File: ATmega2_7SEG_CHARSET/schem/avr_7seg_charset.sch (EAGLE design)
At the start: 19 parts, among them J1 ARDUINO_R3_SHIELD_ICSP-NO_LAB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

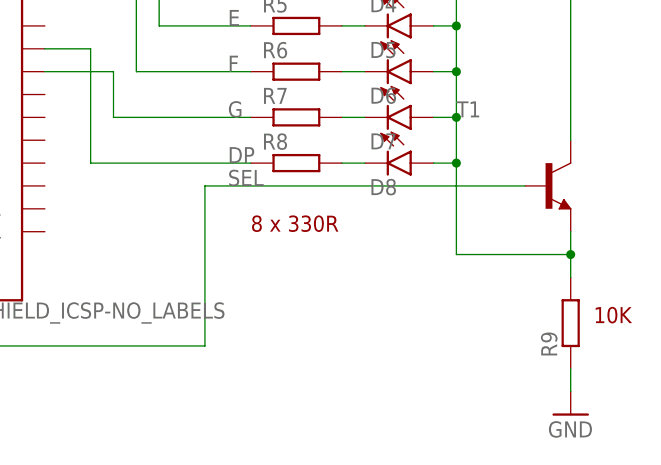
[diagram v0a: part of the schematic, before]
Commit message: corrected the schem
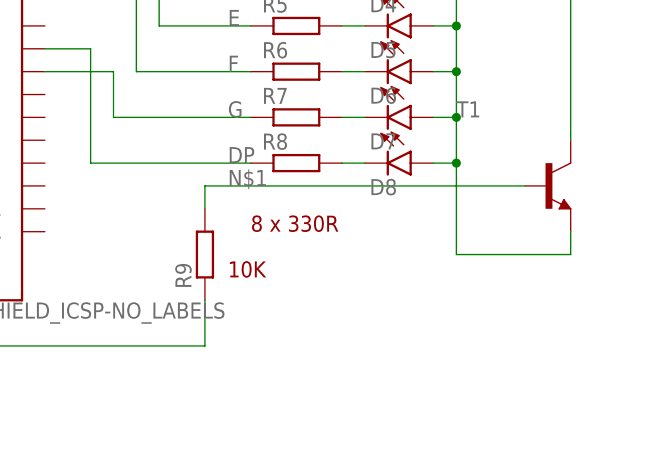
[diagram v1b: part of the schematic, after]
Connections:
- removed net GND: R9.1
- new net N$1: R9.2, T1.B
- net N$10: no longer R9.2
- net SEL: now also R9.1; no longer T1.B
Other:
- moved on the sheet: R9
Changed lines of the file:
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@@
 <part name="T1" library="transistor" deviceset="*-NPN-" device="TO92-EBC"/>
 <part name="SUPPLY1" library="supply2" deviceset="+5V" device=""/>
-<part name="GND1" library="supply1" deviceset="GND" device=""/>
 </parts>
 <sheets>
@@
 <text x="99.06" y="83.82" size="1.778" layer="94">7SEG Common Anode</text>
 <text x="93.98" y="35.56" size="1.778" layer="94">8 x 330R</text>
-<text x="132.08" y="25.4" size="1.778" layer="94">10K</text>
+<text x="91.44" y="30.48" size="1.778" layer="94">10K</text>
 </plain>
 <instances>
@@
 <instance part="R7" gate="G$1" x="99.06" y="48.26"/>
 <instance part="R8" gate="G$1" x="99.06" y="43.18"/>
-<instance part="R9" gate="G$1" x="129.54" y="25.4" rot="R90"/>
+<instance part="R9" gate="G$1" x="88.9" y="33.02" rot="R90"/>
 <instance part="T1" gate="G$1" x="127" y="40.64"/>
 <instance part="SUPPLY1" gate="+5V" x="129.54" y="93.98"/>
-<instance part="GND1" gate="1" x="129.54" y="15.24"/>
 </instances>
 <busses>
@@
 <net name="SEL" class="0">
 <segment>
-<pinref part="T1" gate="G$1" pin="B"/>
-<wire x1="124.46" y1="40.64" x2="88.9" y2="40.64" width="0.1524" layer="91"/>
-<label x="91.44" y="40.64" size="1.778" layer="95"/>
 <pinref part="J1" gate="G$1" pin="A2"/>
 <wire x1="45.72" y1="55.88" x2="43.18" y2="55.88" width="0.1524" layer="91"/>
 <wire x1="43.18" y1="55.88" x2="43.18" y2="22.86" width="0.1524" layer="91"/>
 <wire x1="43.18" y1="22.86" x2="88.9" y2="22.86" width="0.1524" layer="91"/>
-<wire x1="88.9" y1="22.86" x2="88.9" y2="40.64" width="0.1524" layer="91"/>
+<pinref part="R9" gate="G$1" pin="1"/>
+<wire x1="88.9" y1="22.86" x2="88.9" y2="27.94" width="0.1524" layer="91"/>
 </segment>
 </net>
@@
 <junction x="116.84" y="43.18"/>
 <pinref part="T1" gate="G$1" pin="E"/>
-<pinref part="R9" gate="G$1" pin="2"/>
 <wire x1="129.54" y1="35.56" x2="129.54" y2="33.02" width="0.1524" layer="91"/>
-<junction x="129.54" y="33.02"/>
-<wire x1="129.54" y1="33.02" x2="129.54" y2="30.48" width="0.1524" layer="91"/>
 </segment>
 </net>
@@
 </segment>
 </net>
-<net name="GND" class="0">
-<segment>
-<pinref part="R9" gate="G$1" pin="1"/>
-<pinref part="GND1" gate="1" pin="GND"/>
-<wire x1="129.54" y1="20.32" x2="129.54" y2="17.78" width="0.1524" layer="91"/>
-</segment>
-</net>
 <net name="+5V" class="0">
 <segment>
@@
 </segment>
 </net>
+<net name="N$1" class="0">
+<segment>
+<pinref part="T1" gate="G$1" pin="B"/>
+<wire x1="124.46" y1="40.64" x2="88.9" y2="40.64" width="0.1524" layer="91"/>
+<label x="91.44" y="40.64" size="1.778" layer="95"/>
+<pinref part="R9" gate="G$1" pin="2"/>
+<wire x1="88.9" y1="38.1" x2="88.9" y2="40.64" width="0.1524" layer="91"/>
+</segment>
+</net>
